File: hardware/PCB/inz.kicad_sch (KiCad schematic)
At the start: 24 parts, among them J102 ina333, J103 enc, J15 STM32blackpill, J3 USB_C_Receptacle_USB2.0_16P, U101 LMR51430, U3 USBLC6-2SC6

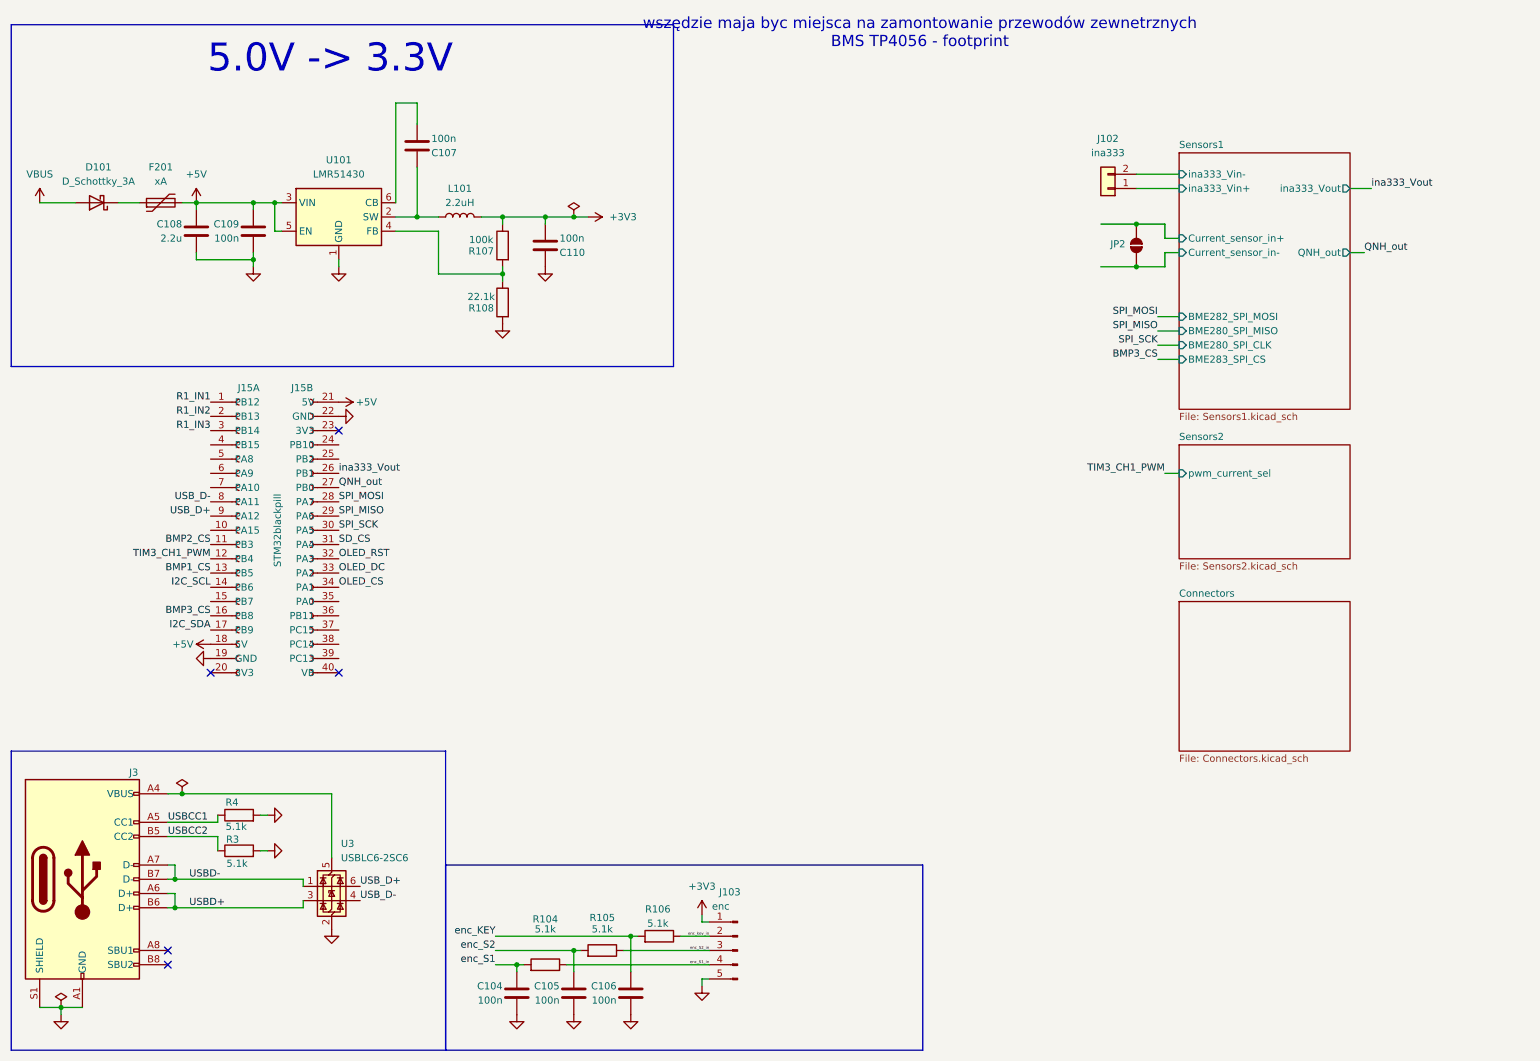
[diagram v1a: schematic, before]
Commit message: pcb sensors
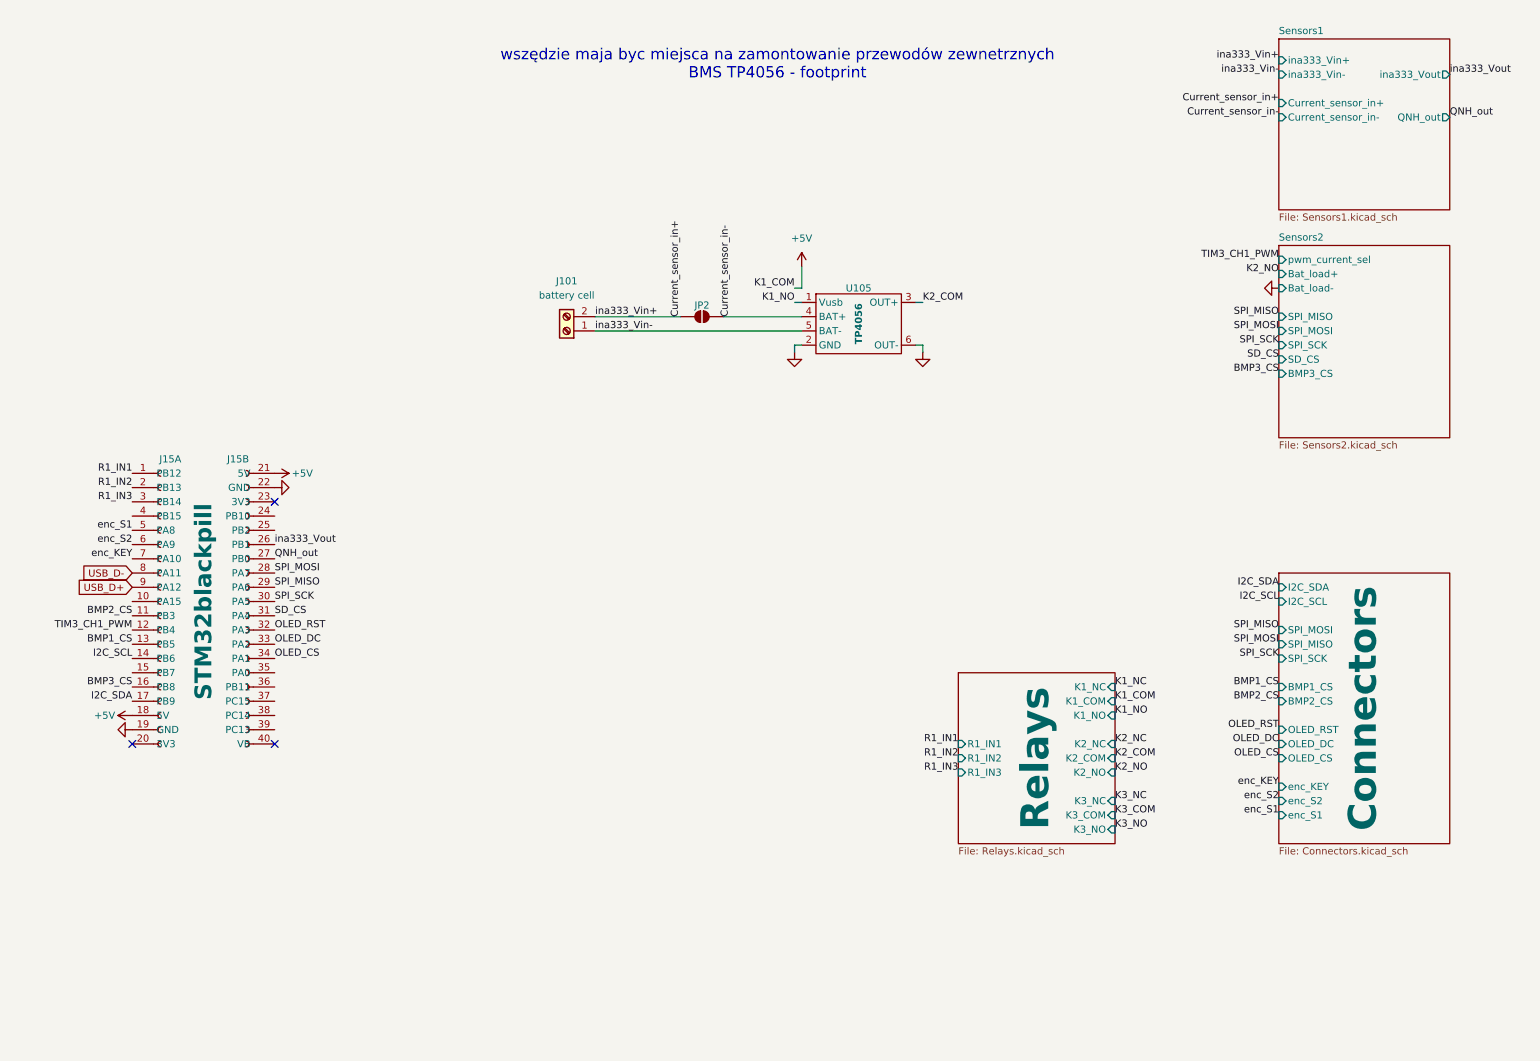
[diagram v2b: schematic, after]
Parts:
- removed C104, C105, C106, C107, C109, C110: 100n, Capacitor_SMD:C_0805_2012Metric, symbol Device:C
- removed C108: 2.2u, Capacitor_SMD:C_0805_2012Metric, symbol Device:C
- removed D101: D_Schottky_3A, Diode_SMD:D_SMA, symbol Device:D_Schottky
- removed F201: xA, Fuse:Fuseholder_Clip-5x20mm_Littelfuse_111_Inline_P20.00x5.00mm_D1.05mm_Horizontal, symbol Device:Polyfuse
- removed J102: ina333, TerminalBlock:TerminalBlock_MaiXu_MX126-5.0-02P_1x02_P5.00mm, symbol Connector_Generic:Conn_01x02
- removed J103: enc, Connector_PinHeader_2.54mm:PinHeader_1x05_P2.54mm_Vertical, symbol Connector:Conn_01x05_Pin
- removed J3: USB_C_Receptacle_USB2.0_16P, Connector_USB:USB_C_Receptacle_GCT_USB4105-xx-A_16P_TopMnt_Horizontal, symbol Connector:USB_C_Receptacle_USB2.0_16P
- removed L101: 2.2uH, Inductor_SMD:L_Sunlord_MWSA0503S, symbol Device:L
- removed R104, R105, R106, R3, R4: 5.1k, Resistor_SMD:R_0805_2012Metric, symbol Device:R
- removed R107: 100k, Resistor_SMD:R_0805_2012Metric, symbol Device:R
- removed R108: 22.1k, Resistor_SMD:R_0805_2012Metric, symbol Device:R
- removed U101: LMR51430, Package_TO_SOT_SMD:SOT-23-6, symbol Regulator_Switching:LMR51430
- removed U3: USBLC6-2SC6, Package_TO_SOT_SMD:SOT-23-6, symbol Power_Protection:USBLC6-2SC6
- added J101: battery cell, symbol Connector:Screw_Terminal_01x02
- added U105: TP4056, symbol footprints:TP4056
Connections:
- net GND: now also U105.2 (GND), U105.6 (OUT-)
- net enc_KEY: now also J15.7 (PA10)
- net enc_S1: now also J15.5 (PA8)
- net enc_S2: now also J15.6 (PA9)
- net Sensors1/Current_sensor_in+ renamed Current_sensor_in+
- net Current_sensor_in+: now also J101.2 (Pin_2)
- net Sensors1/Current_sensor_in- renamed Current_sensor_in-
- net Current_sensor_in-: now also U105.4 (BAT+)
- new net K1_NO: U105.1 (Vusb)
- new net K2_COM: U105.3 (OUT+)
- new net ina333_Vin-: J101.1 (Pin_1), U105.5 (BAT-)
- no-connect marks 5 -> 3
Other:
- added sheet Relays (Relays.kicad_sch)
- sheet Connectors ports: added BMP1_CS, BMP2_CS, I2C_SCL, I2C_SDA, OLED_CS, OLED_DC, OLED_RST, SPI_MISO, SPI_MOSI, SPI_SCK, enc_KEY, enc_S1, enc_S2; removed none
- sheet Sensors1 ports: added none; removed BME280_SPI_CLK, BME280_SPI_MISO, BME282_SPI_MOSI, BME283_SPI_CS
- sheet Sensors2 ports: added BMP3_CS, Bat_load+, Bat_load-, SD_CS, SPI_MISO, SPI_MOSI, SPI_SCK; removed none
- note removed: "5.0V -> 3.3V"
- moved on the sheet: J15A, J15B, JP2
